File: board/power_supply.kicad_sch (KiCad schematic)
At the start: 53 parts, among them J1 USB, J2 LiPo, U1 IP5303, U10 MAX809T, U2 TPS562201, U3 RT9069, U4 TPS55340

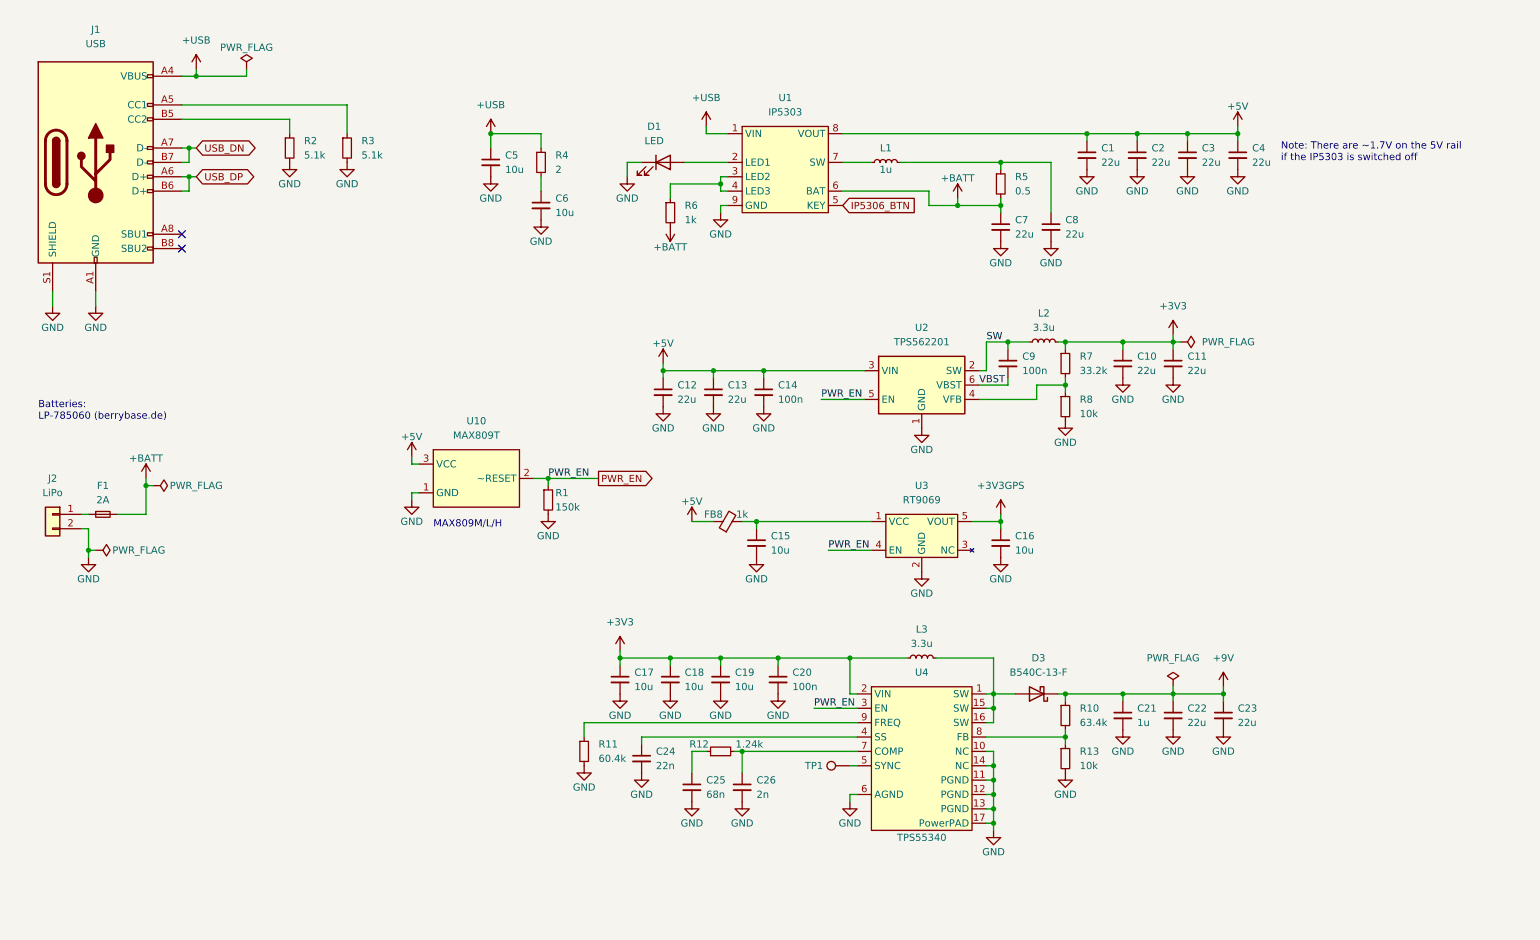
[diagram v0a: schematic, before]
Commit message: Hardware Revision
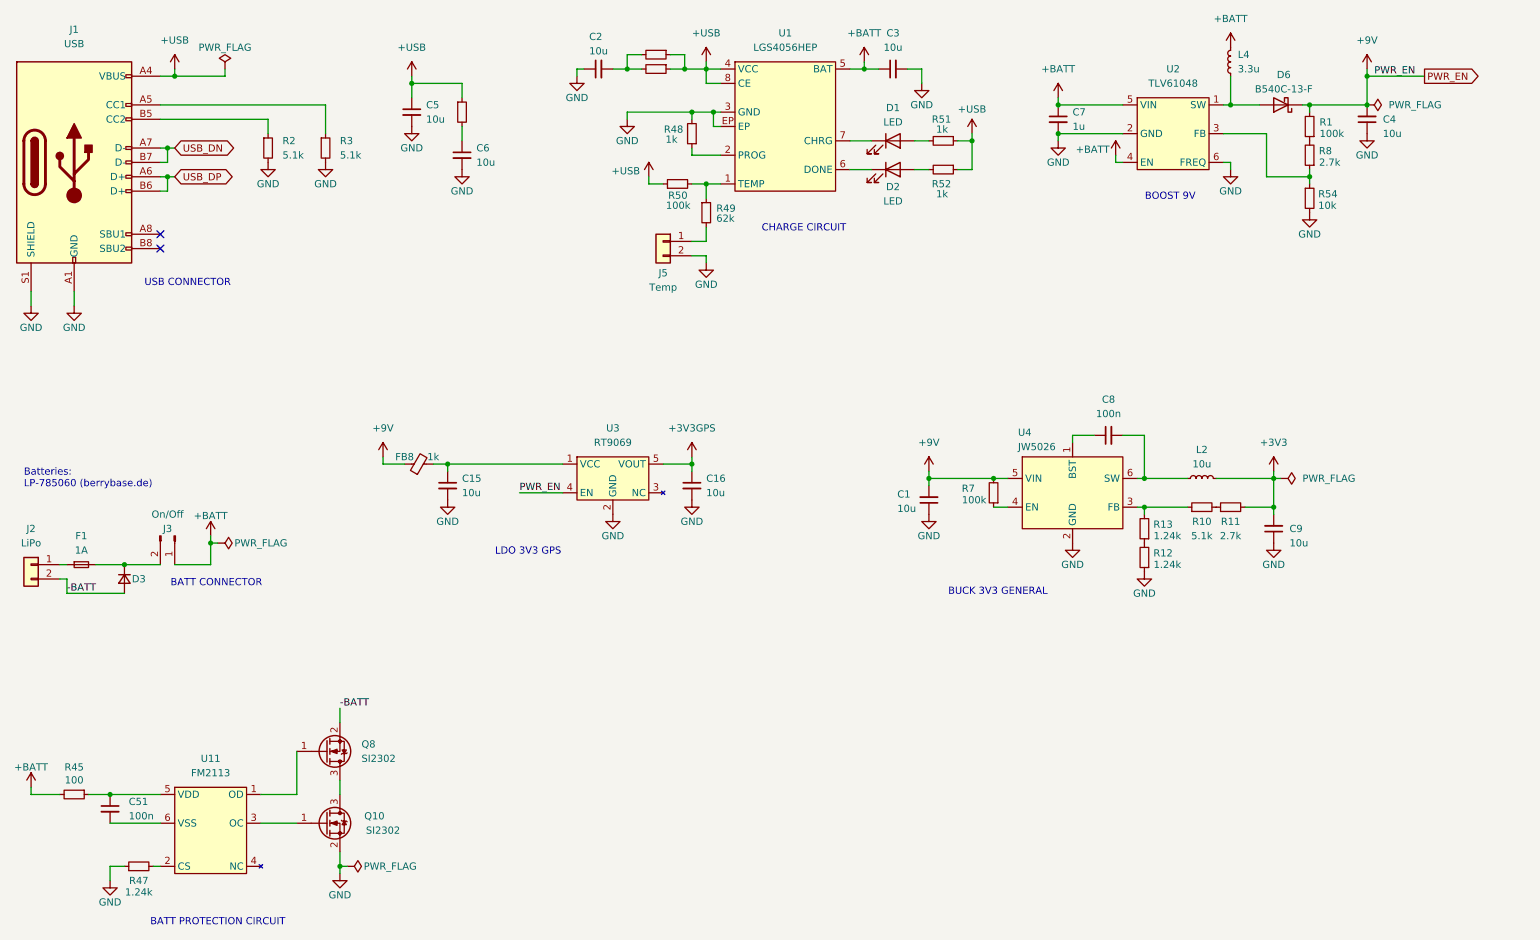
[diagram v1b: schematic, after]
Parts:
- removed C10, C11, C12, C13, C22, C23: 22u, Capacitor_SMD:C_1206_3216Metric, symbol Device:C_Small
- removed C14, C20: 100n, Capacitor_SMD:C_0603_1608Metric, symbol Device:C_Small
- removed C17, C18, C19: 10u, Capacitor_SMD:C_0603_1608Metric, symbol Device:C_Small
- removed C21: 1u, Capacitor_SMD:C_0603_1608Metric, symbol Device:C_Small
- removed C24: 22n, Capacitor_SMD:C_0603_1608Metric, symbol Device:C_Small
- removed C25: 68n, Capacitor_SMD:C_0603_1608Metric, symbol Device:C_Small
- removed C26: 2n, Capacitor_SMD:C_0603_1608Metric, symbol Device:C_Small
- removed D3: B540C-13-F, Diode_SMD:D_SMC, symbol Device:D_Schottky
- removed L1: 1u, Inductor_SMD:L_Vishay_IFSC-1515AH_4x4x1.8mm, symbol Device:L_Small
- removed L3: 3.3u, Inductor_SMD:L_Sunlord_MWSA0503S, symbol Device:L_Small
- removed TP1: TestPoint, TestPoint:TestPoint_Pad_1.0x1.0mm, symbol Connector:TestPoint
- removed U1: IP5303, Package_SO:HSOP-8-1EP_3.9x4.9mm_P1.27mm_EP2.3x2.3mm, symbol OBSPro:IP5303
- removed U10: MAX809T, Package_TO_SOT_SMD:SOT-23-3, symbol OBSPro:MAX809
- removed U2: TPS562201, Package_TO_SOT_SMD:SOT-23-6, symbol Regulator_Switching:TPS562200
- removed U4: TPS55340, Package_DFN_QFN:VQFN-16-1EP_3x3mm_P0.5mm_EP1.68x1.68mm, symbol OBSPro:TPS55340R
- added C51: 100n, Capacitor_SMD:C_0603_1608Metric, symbol Device:C_Small
- added D2: LED, LED_SMD:LED_0603_1608Metric, symbol Device:LED
- added D3: D_Small, Diode_SMD:D_SOD-123F, symbol Device:D_Small
- added D6: B540C-13-F, Diode_SMD:D_SMC, symbol Device:D_Schottky
- added J3: On/Off, OpenBikeSensor:Connector_1x02_Switch, symbol Connector:Conn_01x02_Male
- added J5: Temp, Connector_JST:JST_PH_S2B-PH-K_1x02_P2.00mm_Horizontal, symbol Connector_Generic:Conn_01x02
- added L4: 3.3u, symbol Device:L_Small
- added Q10, Q8: SI2302, Package_TO_SOT_SMD:SOT-23, symbol Device:Q_NMOS_GSD
- added R45: 100, Resistor_SMD:R_0603_1608Metric, symbol Device:R_Small
- added R47: 1.24k, Resistor_SMD:R_0603_1608Metric, symbol Device:R_Small
- added R48, R51, R52: 1k, Resistor_SMD:R_0603_1608Metric, symbol Device:R_Small
- added R49: 62k, Resistor_SMD:R_0603_1608Metric, symbol Device:R_Small
- added R50: 100k, Resistor_SMD:R_0603_1608Metric, symbol Device:R_Small
- added R54: 10k, Resistor_SMD:R_0603_1608Metric, symbol Device:R_Small
- added U1: LGS4056HEP, Package_SO:SOP-8-1EP_4.57x4.57mm_P1.27mm_EP4.57x4.45mm, symbol OBSPro:LGS4056HEP
- added U11: FM2113, Package_TO_SOT_SMD:SOT-23-6, symbol OBSPro:FM2113
- added U2: TLV61048, Package_TO_SOT_SMD:SOT-23-6, symbol OBSPro:TLV61048
- added U4: JW5026, Package_TO_SOT_SMD:SOT-23-6, symbol OBSPro:JW5026
- C1, C2, C3, C4: value 22u -> 10u; footprint Capacitor_SMD:C_1206_3216Metric -> Capacitor_SMD:C_0603_1608Metric; JLC_BasicPart no -> yes; JLC_PN C5672 -> C19702; JLC_Price1 (none) -> 0.062; JLC_Price10 0.0217 -> 0.0052; JLC_Price100 (none) -> 0.0031; JLC_Price1000 (none) -> 0.0029; MPN CL31A226KPHNNNE -> CL10A106KP8NNNC; kicost:JLC:pricing 1: USD 0.0192; 150: USD 0.0186 -> 1: USD 0.062; 10: USD 0.0062; 100: USD 0.0031; 1000: USD 0.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
- C7: value 22u -> 1u; footprint Capacitor_SMD:C_1206_3216Metric -> Capacitor_SMD:C_0603_1608Metric; JLC_BasicPart no -> yes; JLC_PN C5672 -> C15849; JLC_Price1 (none) -> 0.056; JLC_Price10 0.0217 -> 0.0051; JLC_Price100 (none) -> 0.0028; JLC_Price1000 (none) -> 0.0027; MPN CL31A226KPHNNNE -> CL10A105KB8NNNC; kicost:JLC:pricing 1: USD 0.0192; 150: USD 0.0186 -> 1: USD 0.056; 10: USD 0.0056; 100: USD 0.0028; 1000: USD 0.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
- C8: value 22u -> 100n; footprint Capacitor_SMD:C_1206_3216Metric -> Capacitor_SMD:C_0603_1608Metric; JLC_BasicPart no -> yes; JLC_PN C5672 -> C14663; JLC_Price1 (none) -> 0.042; JLC_Price10 0.0217 -> 0.0021; JLC_Price100 (none) -> 0.0021; JLC_Price1000 (none) -> 0.0014; MPN CL31A226KPHNNNE -> CC0603KRX7R9BB104; Manufacturer Samsung Electro-Mechanics -> YAGEO; kicost:JLC:pricing 1: USD 0.0192; 150: USD 0.0186 -> 1: USD 0.0020; 200: USD 0.0016; 800: USD 0.0013; 1600: USD 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
- C9: value 100n -> 10u; JLC_PN C14663 -> C19702; JLC_Price1 0.042 -> 0.062; JLC_Price10 0.0021 -> 0.0052; JLC_Price100 0.0021 -> 0.0031; JLC_Price1000 0.0014 -> 0.0029; MPN CC0603KRX7R9BB104 -> CL10A106KP8NNNC; Manufacturer YAGEO -> Samsung Electro-Mechanics; kicost:JLC:pricing 1: USD 0.0020; 200: USD 0.0016; 800: USD 0.0013; 1600: USD 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 -> 1: USD 0.062; 10: USD 0.0062; 100: USD 0.0031; 1000: USD 0.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
- F1: value 2A -> 1A; JLC_PN C187605 -> C151139; MPN 0467002.NRHF -> 0467001.NRHF
- L2: value 3.3u -> 10u; footprint Inductor_SMD:L_Vishay_IFSC-1515AH_4x4x1.8mm -> (none); JLC_BasicPart no -> (none); JLC_PN C98362 -> (none); JLC_Price10 0.0766 -> (none); MPN WPN4020H3R3MT -> FNR6045S100MT; Manufacturer Sunlord -> cjiang
- R1: value 150k -> 100k; JLC_BasicPart (none) -> yes; JLC_PN C22807 -> (none); MPN 0603WAF1503T5E -> 0603WAF1003T5E
- R10: value 63.4k -> 5.1k; JLC_BasicPart no -> yes; JLC_PN C23093 -> C23186; JLC_Price10 (none) -> 0.0009; MPN 0603WAF6342T5E -> 0603WAF5101T5E; PCBA (none) -> yes; kicost:JLC:pricing (none) -> 1: USD 0.0009; 200: USD 0.0007; 1000: USD 0.0006; 10000: US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
- R11: value 60.4k -> 2.7k; JLC_BasicPart no -> yes; JLC_PN C23089 -> C13167; MPN 0603WAF6042T5E -> 0603WAF2701T5E
- R13: value 10k -> 1.24k; JLC_BasicPart yes -> no; JLC_PN C25804 -> C25956; JLC_Price10 0.0013 -> (none); MPN 0603WAF1002T5E -> 0603WAF1241T5E; Manufacturer UNI-ROYAL(Uniroyal Elec) -> UNI-ROYAL(Uniroyal Elec)
- R5: value 0.5 -> 2; JLC_BasicPart no -> yes; JLC_PN C45312 -> C22977; JLC_Price10 0.0025 -> 0.0012; MPN 0603WAF500LT5E -> 0603WAF200KT5E; kicost:JLC:pricing 1: USD 0.0044; 200: USD 0.0037; 1000: USD 0.0033; 2000: USD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 -> 1: USD 0.0014; 200: USD 0.0011; 1000: USD 0.0009
- R6: value 1k -> 2; JLC_PN C21190 -> C22977; JLC_Price10 0.0005 -> 0.0012; MPN 0603WAF1001T5E -> 0603WAF200KT5E; kicost:JLC:pricing 1: USD 0.0005; 200: USD 0.0004 -> 1: USD 0.0014; 200: USD 0.0011; 1000: USD 0.0009
- R7: value 33.2k -> 100k; JLC_BasicPart no -> yes; JLC_PN C23003 -> (none); JLC_Price10 0.0009 -> (none); MPN 0603WAF3322T5E -> 0603WAF1003T5E; PCBA (none) -> yes
- R8: value 10k -> 2.7k; JLC_PN C25804 -> C13167; JLC_Price10 0.0013 -> (none); MPN 0603WAF1002T5E -> 0603WAF2701T5E
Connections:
- net VBST is gone; now on net +3V3: C9.2
- net +3V3: now also R11.2; no longer R7.1
- net +9V: now also C1.2, C4.2, FB8.1, R1.2, R7.2, U3.4 (EN), D6.1 (K), U4.5 (VIN); no longer R10.1
- net +BATT: now also C3.1, J3.1 (Pin_1), L4.2, R45.2, U1.5 (BAT), U2.4 (EN), U2.5 (VIN); no longer F1.2, R5.2, R6.2
- net +USB: now also R5.1, R6.1, R50.1, R51.1, R52.1, U1.4 (VCC), U1.8 (CE)
- net GND: now also C1.1, C2.1, C4.1, C9.1, R12.1, J5.2 (Pin_2), Q10.2 (S), R47.1, R48.2, R54.2, U1.3 (GND), U1.EP, U2.2 (GND), U2.6 (FREQ), U4.2 (GND); no longer C1.2, C2.2, C4.2, C8.2, D1.1 (K), J2.2 (Pin_2), R1.2, R11.2, R13.2, R8.2
- net at R12.2: now also R13.1
- net at C8.1: now also U4.1 (BST); no longer R5.1
- net at R10.2: now also R11.1; no longer R13.1
- net at D1.2 (A): now also R51.2
- net at R8.1: now also R54.1, U2.3 (FB); no longer R7.2
- removed net +5V: C1.1, C2.1, C3.1, C4.1, FB8.1
- net PWR_EN: no longer names the net of R1.1
- net PWR_EN: now also R8.2; no longer U3.4 (EN)
- net SW: no longer names the net of L2.1
- net SW: now also C8.2, U4.6 (SW); no longer C9.1
- new net: Q8.1 (G), U11.1 (OD)
- new net: Q10.3 (D), Q8.3 (D)
- new net: R49.1, R50.2, U1.1 (TEMP)
- new net: Q10.1 (G), U11.3 (OC)
- new net: R48.1, U1.2 (PROG)
- new net: D2.1 (K), U1.6 (DONE)
- new net: D1.1 (K), U1.7 (CHRG)
- new net: C51.1, R45.1, U11.5 (VDD)
- new net: C51.2, U11.6 (VSS)
- new net: J5.1 (Pin_1), R49.2
- new net: D3.1 (K), F1.2, J3.2 (Pin_2)
- new net: C2.2, R5.2, R6.2
- new net: R47.2, U11.2 (CS)
- new net: D6.2 (A), L4.1, U2.1 (SW)
- new net: D2.2 (A), R52.2
- new net: R7.1, U4.4 (EN)
- new net: R10.1, R13.2, U4.3 (FB)
- new net -BATT: D3.2 (A), J2.2 (Pin_2), Q8.2 (S)
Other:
- note added: "BATT CONNECTOR"
- note added: "BATT PROTECTION CIRCUIT"
- note added: "BOOST 9V"
- note added: "BUCK 3V3 GENERAL"
- note added: "CHARGE CIRCUIT"
- note added: "LDO 3V3 GPS"
- note added: "USB CONNECTOR"
- note removed: "MAX809M/L/H"
- note removed: "Note: There are ~1.7V on the 5V rail if the IP5303 is switched off"
- moved on the sheet: C15, C16, C5, C6, D1, F1, FB8, J1, J2, R2, R3, U3
